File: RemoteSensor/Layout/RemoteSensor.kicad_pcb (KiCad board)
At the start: 2 copper layers, 50.8 x 50.8 mm, 68 parts, among them J1 USB_B_Micro, J2 BATT_CONN, J3 LCD_HEADER, J4 PRG_HEADER, Q1 2N7002, Q2 2N7002, Q3 2N7002, Q4 MMBT2222A-TP, Q5 MMBT2222A-TP, SW1 BTN_RST, SW2 SW_Push, U1 MCP73831-2-OT, U10 FT231XS, U2 LM3671MF, U3 BD48ExxG, U4 BD48ExxG, U5 LM3671MF, U6 74LVC2G02, U7 ESP-12F, U8 LM50CIM3, U9 MCP23008-E_P

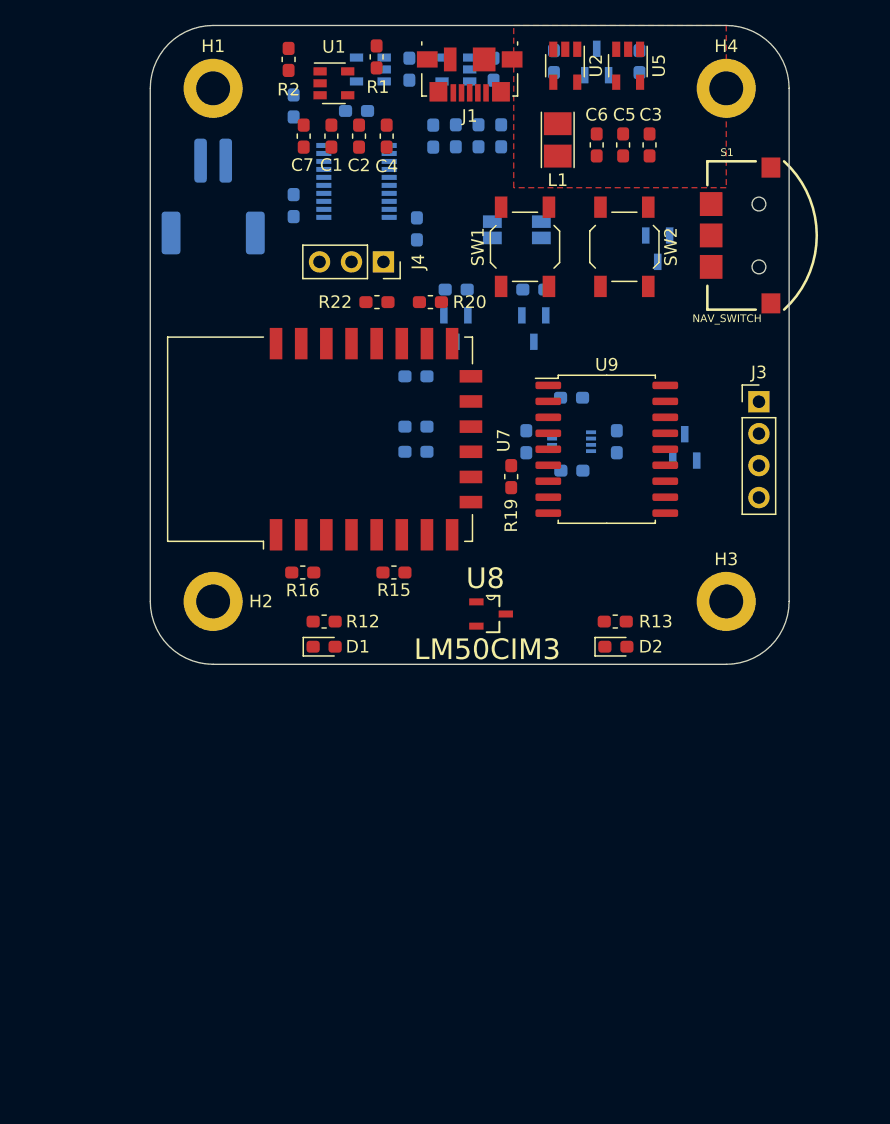
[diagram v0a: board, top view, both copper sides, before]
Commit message: Update PCB layout
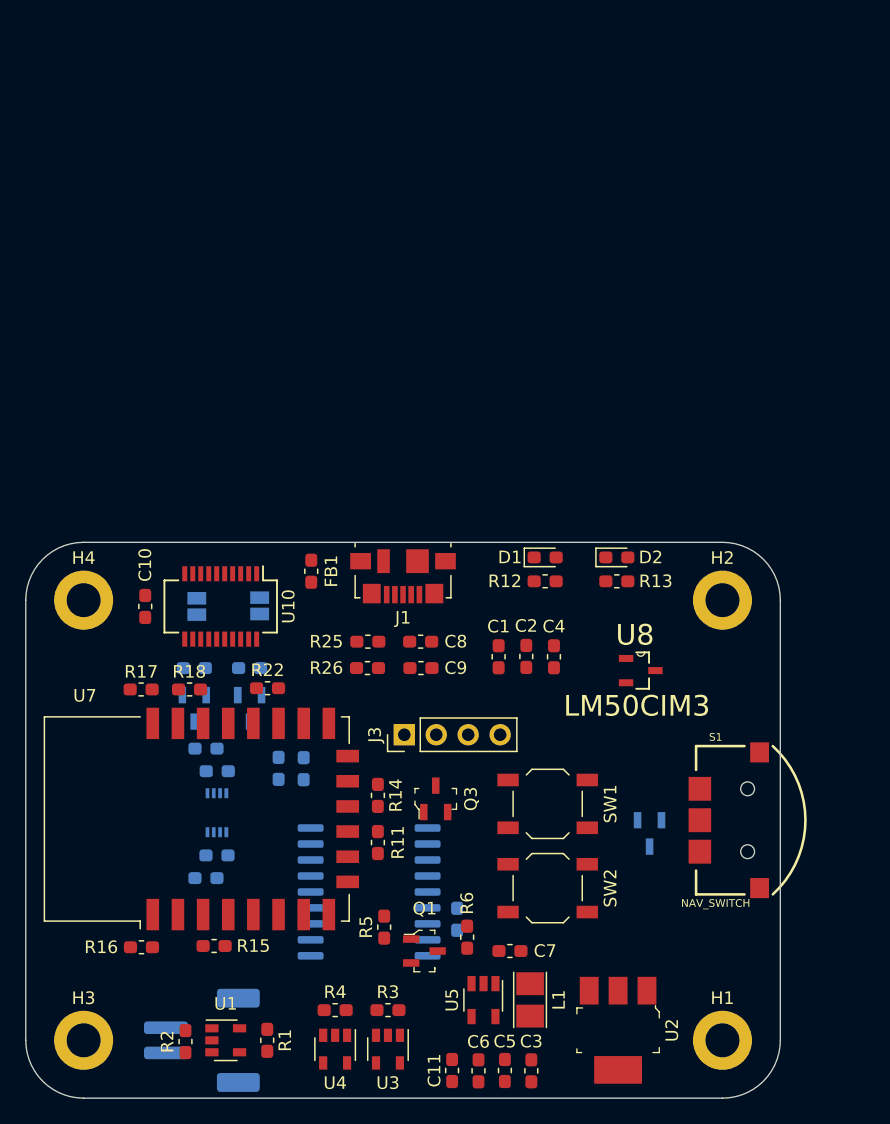
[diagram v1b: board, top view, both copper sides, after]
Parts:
- removed J4: PRG_HEADER, Connector_PinSocket_2.54mm:PinSocket_1x03_P2.54mm_Vertical
- added C11: 10u, Capacitor_SMD:C_0603_1608Metric_Pad1.05x0.95mm_HandSolder, F.Cu at (138.3, 147.4)
- C10, C8, C9, FB1, Q1, Q3, R11, R14, R17, R18, R25, R26, R3, R4, R5, R6, U10, U3, U4: moved to F.Cu
- R19, R20, U9: moved to B.Cu
- U2: value LM3671MF -> LD1117S33CTR; footprint Package_TO_SOT_SMD:TSOT-23-5 -> digikey-footprints:SOT-223
- moved H1 85.9 mm to (159.8, 145.0)
- moved R1 78.7 mm to (123.6, 145.0), turned to 270 degrees
- moved R2 78.5 mm to (117.1, 145.1), turned to 90 degrees
- moved U4 78.5 mm to (129.0, 145.7), turned to 270 degrees
- moved U3 77.9 mm to (133.2, 145.7), turned to 270 degrees
- moved U2 76.8 mm to (151.5, 144.2), turned to 180 degrees
- moved U1 76.6 mm to (120.3, 145.0)
- moved R4 75.9 mm to (129.0, 142.6), turned to 0 degrees
- moved U5 75.2 mm to (140.8, 141.8)
- moved R3 74.8 mm to (133.2, 142.6), turned to 0 degrees
- moved C3 74.2 mm to (144.6, 147.4), turned to 270 degrees
- moved C6 74.2 mm to (140.4, 147.4), turned to 270 degrees
- moved C5 74.2 mm to (142.5, 147.4), turned to 270 degrees
- moved Q1 72.0 mm to (136.1, 137.9), turned to 0 degrees
- moved R5 71.8 mm to (132.9, 136.0)
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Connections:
- U2 pad 1: V_USB -> GND
- U2 pad 2: GND -> 3.3V
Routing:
- removed copper zone on F.Cu, net GND
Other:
- board size 50.8 x 50.8 mm -> 60 x 44.2 mm
- rule pad_to_mask_clearance: 0.051 -> 0

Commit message: Generate routing
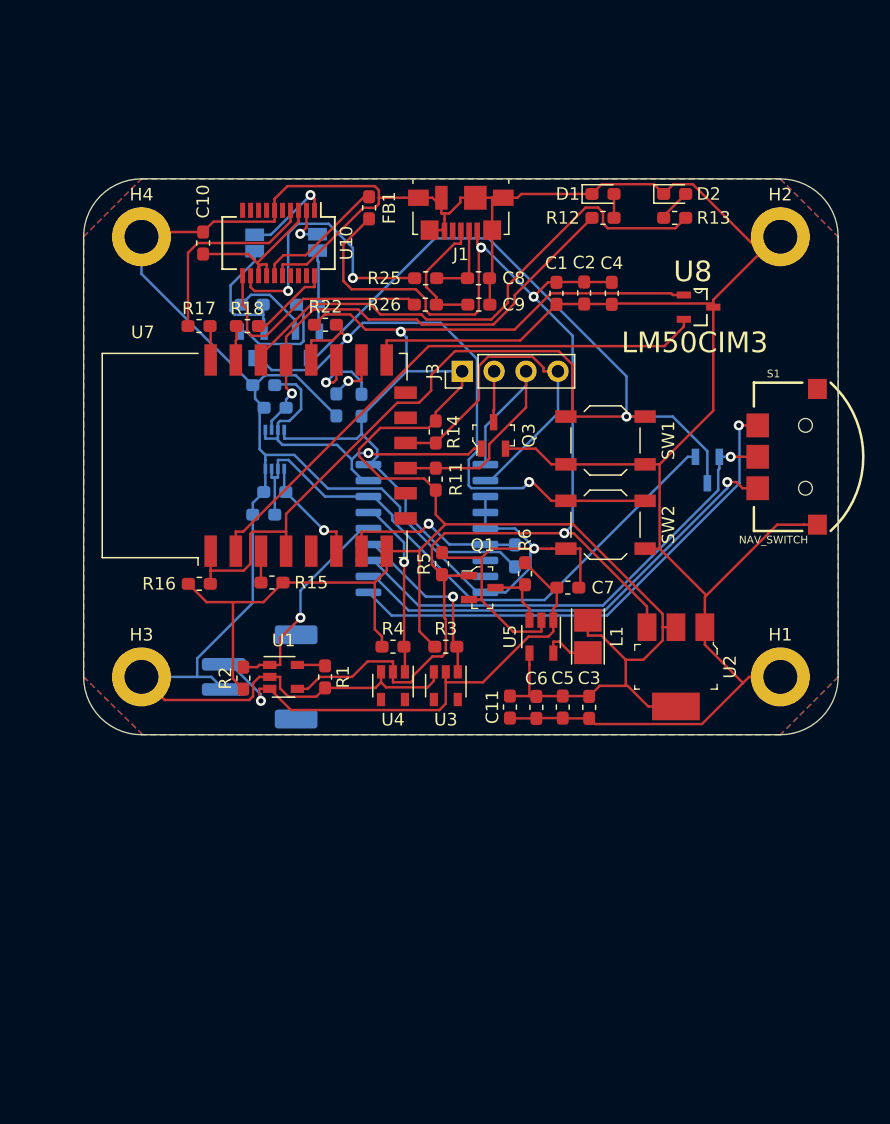
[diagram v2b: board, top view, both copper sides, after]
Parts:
- moved C9 29.3 mm to (140.4, 86.5)
- moved R12 29.3 mm to (150.3, 79.6)
- moved R19 29.3 mm to (143.3, 106.5)
- moved R26 29.3 mm to (136.2, 86.5)
- moved C1 29.3 mm to (146.6, 85.6)
- moved C10 29.3 mm to (118.5, 81.6)
- moved C11 29.3 mm to (142.9, 118.5)
- moved C3 29.3 mm to (149.2, 118.5)
- moved C4 29.3 mm to (151.0, 85.6)
- moved C5 29.3 mm to (147.1, 118.5)
- moved C6 29.3 mm to (145.0, 118.5)
- moved C7 29.3 mm to (147.5, 109.0)
- moved FB1 29.3 mm to (131.7, 78.8)
- moved H1 29.3 mm to (164.4, 116.1)
- moved H2 29.3 mm to (164.4, 81.1)
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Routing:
- net GND: track 0.00 -> 347.4 mm, vias 0 -> 1
- net 3.3V: track 0.00 -> 191.4 mm, vias 0 -> 1
- net V_USB: track 0.00 -> 105.8 mm, vias 0 -> 3
- net RST: track 0.00 -> 101.2 mm, vias 0 -> 1
- net FLASH: track 0.00 -> 51.9 mm, vias 0 -> 2
- net SLEEP_STS: track 0.00 -> 48.3 mm
- net /Processor/TEMP_PIN: track 0.00 -> 44.5 mm
- net BATT_PIN: track 0.00 -> 42.4 mm
- net V_BATT: track 0.00 -> 40.9 mm, vias 0 -> 1
- net UP_BTN: track 0.00 -> 40.7 mm, vias 0 -> 1
- net CENTER_BTN: track 0.00 -> 38.8 mm, vias 0 -> 1
- net HB_PIN: track 0.00 -> 37.9 mm, vias 0 -> 1
- net DOWN_BTN: track 0.00 -> 36.8 mm, vias 0 -> 1
- net WAKE_STS: track 0.00 -> 29.0 mm, vias 0 -> 1
- net /Processor/SDA: track 0.00 -> 28.5 mm
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- added copper zone on B.Cu, net GND
- added copper zone on F.Cu, net GND
